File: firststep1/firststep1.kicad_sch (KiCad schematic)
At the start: 0 parts

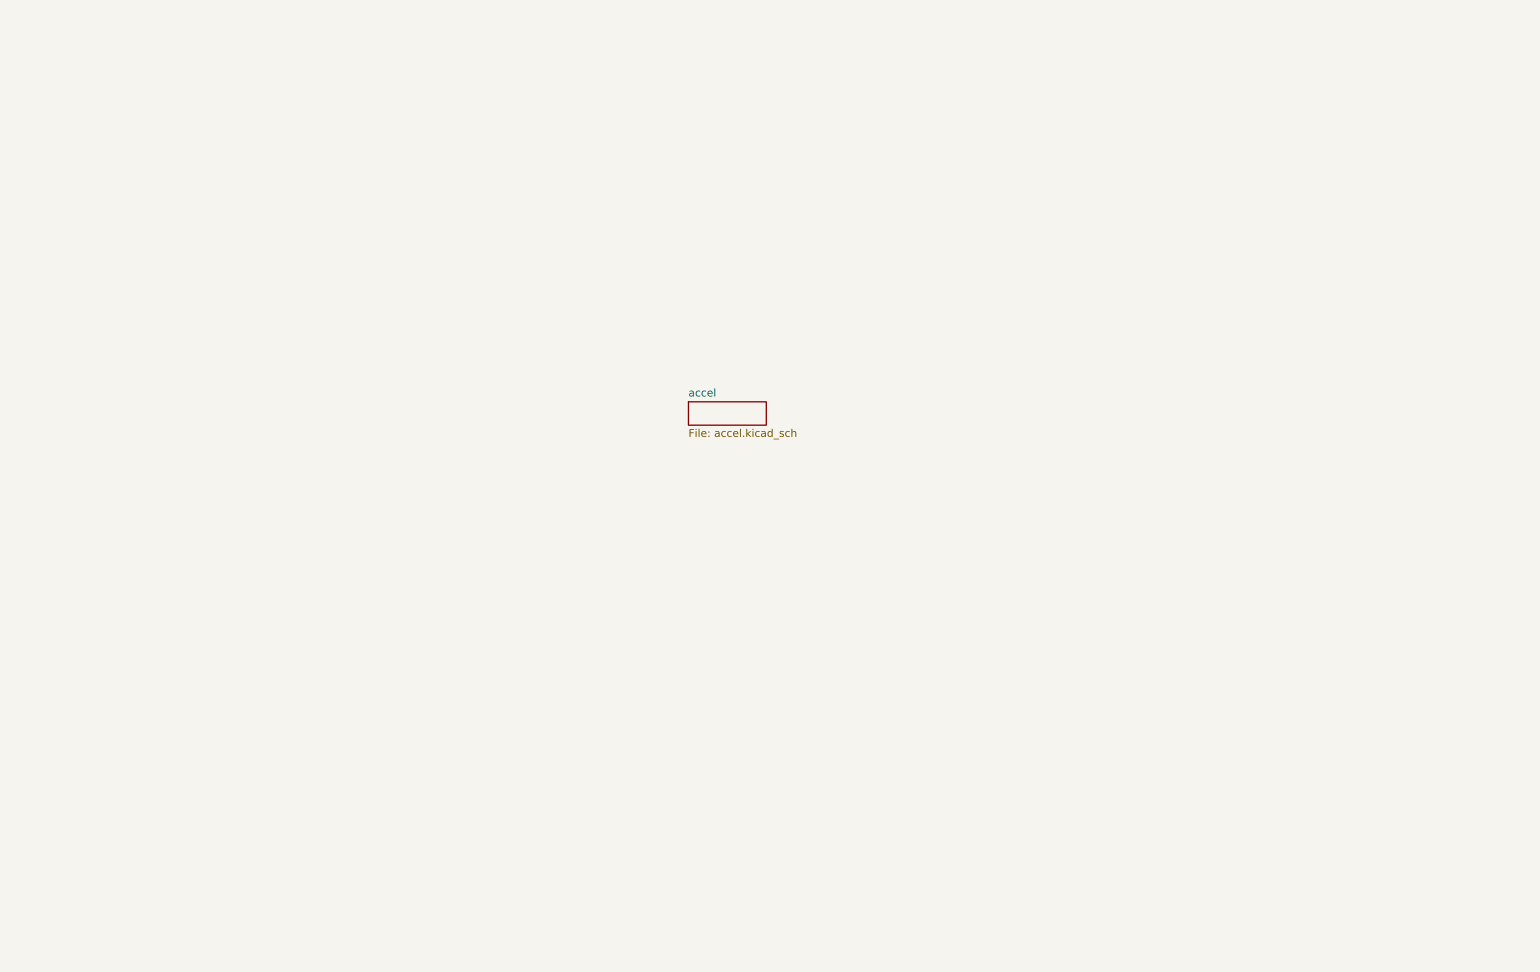
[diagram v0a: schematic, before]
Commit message: many changes
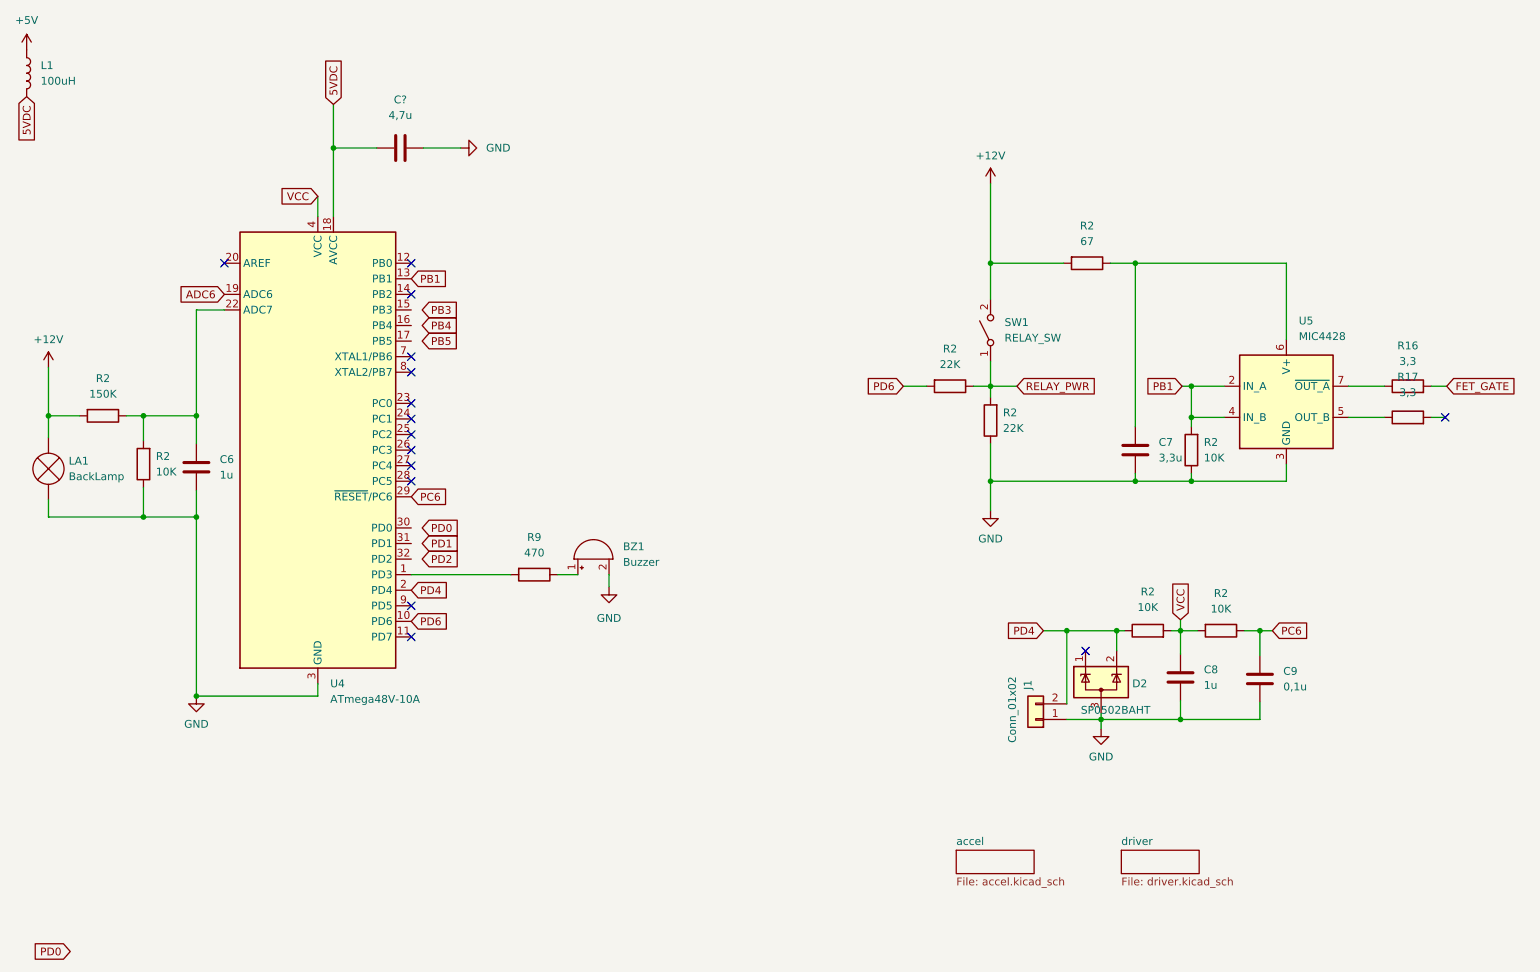
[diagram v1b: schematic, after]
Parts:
- added BZ1: Buzzer, Buzzer_Beeper:Buzzer_12x9.5RM7.6, symbol Device:Buzzer
- added C6, C8: 1u, Capacitor_THT:C_Disc_D3.0mm_W2.0mm_P2.50mm, symbol Device:C
- added C7: 3,3u, Capacitor_THT:C_Disc_D3.0mm_W2.0mm_P2.50mm, symbol Device:C
- added C9: 0,1u, Capacitor_THT:C_Disc_D3.0mm_W2.0mm_P2.50mm, symbol Device:C
- added C?: 4,7u, Capacitor_THT:C_Disc_D3.0mm_W2.0mm_P2.50mm, symbol Device:C
- added D2: SP0502BAHT, Package_TO_SOT_SMD:SOT-23, symbol Power_Protection:SP0502BAHT
- added J1: Conn_01x02, Connector_Wago:Wago_734-162_1x02_P3.50mm_Horizontal, symbol Connector_Generic:Conn_01x02
- added L1: 100uH, symbol Device:L
- added LA1: BackLamp, symbol Device:Lamp
- added R16, R17: 3,3, Resistor_THT:R_Axial_DIN0204_L3.6mm_D1.6mm_P7.62mm_Horizontal, symbol Device:R
- added R2 (x8): 330, R_Axial_DIN0207_L6.3mm_D2.5mm_P7.62mm_Horizontal, symbol Device:R
- added R9: 470, Resistor_THT:R_Axial_DIN0207_L6.3mm_D2.5mm_P7.62mm_Horizontal, symbol Device:R
- added SW1: RELAY_SW, symbol Switch:SW_SPST
- added U4: ATmega48V-10A, Package_QFP:TQFP-32_7x7mm_P0.8mm, symbol MCU_Microchip_ATmega:ATmega48V-10A
- added U5: MIC4428, Package_DIP:DIP-8_W7.62mm_Socket, symbol Driver_FET:MIC4428
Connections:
- new net: C6.1, R2.1, R2.2, U4.22 (ADC7)
- new net: R17.1, U5.5 (OUT_B)
- new net: C7.1, R2.1, U5.6 (V+)
- new net: R16.1, U5.7 (~{OUT_A})
- new net: BZ1.1 (-), R9.1
- new net: R9.2, U4.1 (PD3)
- new net +12V: LA1.2 (+), R2.2, R2.2, SW1.2 (B)
- new net +5V: L1.1
- new net 5VDC: C?.1, L1.2, U4.18 (AVCC)
- new net ADC6: U4.19 (ADC6)
- new net FET_GATE: R16.2
- new net GND: BZ1.2 (+), C6.2, C7.2, C8.2, C9.1, C?.2, D2.3 (A), J1.1 (Pin_1), LA1.1 (-), R2.1, R2.1, R2.1, U4.21 (GND), U4.3 (GND), U4.5 (GND), U5.3 (GND)
- new net PB1: R2.2, U4.13 (PB1), U5.2 (IN_A), U5.4 (IN_B)
- new net PC6: C9.2, R2.1, U4.29 (~{RESET}/PC6)
- new net PD4: D2.2 (K), J1.2 (Pin_2), R2.1, U4.2 (PD4)
- new net PD6: R2.2, U4.10 (PD6)
- new net RELAY_PWR: R2.1, R2.2, SW1.1 (A)
- new net VCC: C8.1, R2.2, R2.2, U4.4 (VCC), U4.6 (VCC)
- no-connect marks 0 -> 15
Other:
- added sheet driver (driver.kicad_sch)
